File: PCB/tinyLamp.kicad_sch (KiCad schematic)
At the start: 54 parts, among them J1 USB_B_Mini, J2 Conn_02x03_Odd_Even, Q1 Q_NPN_BCE, Q2 Q_NPN_BCE, Q3 Q_NPN_BCE, Q4 Q_NPN_BCE, SW1 SW_Push, SW2 SW_Push, SW3 SW_Push, U1 TP4056, U2 ATtiny13A-SS, X1 BATT+, X2 BATT-

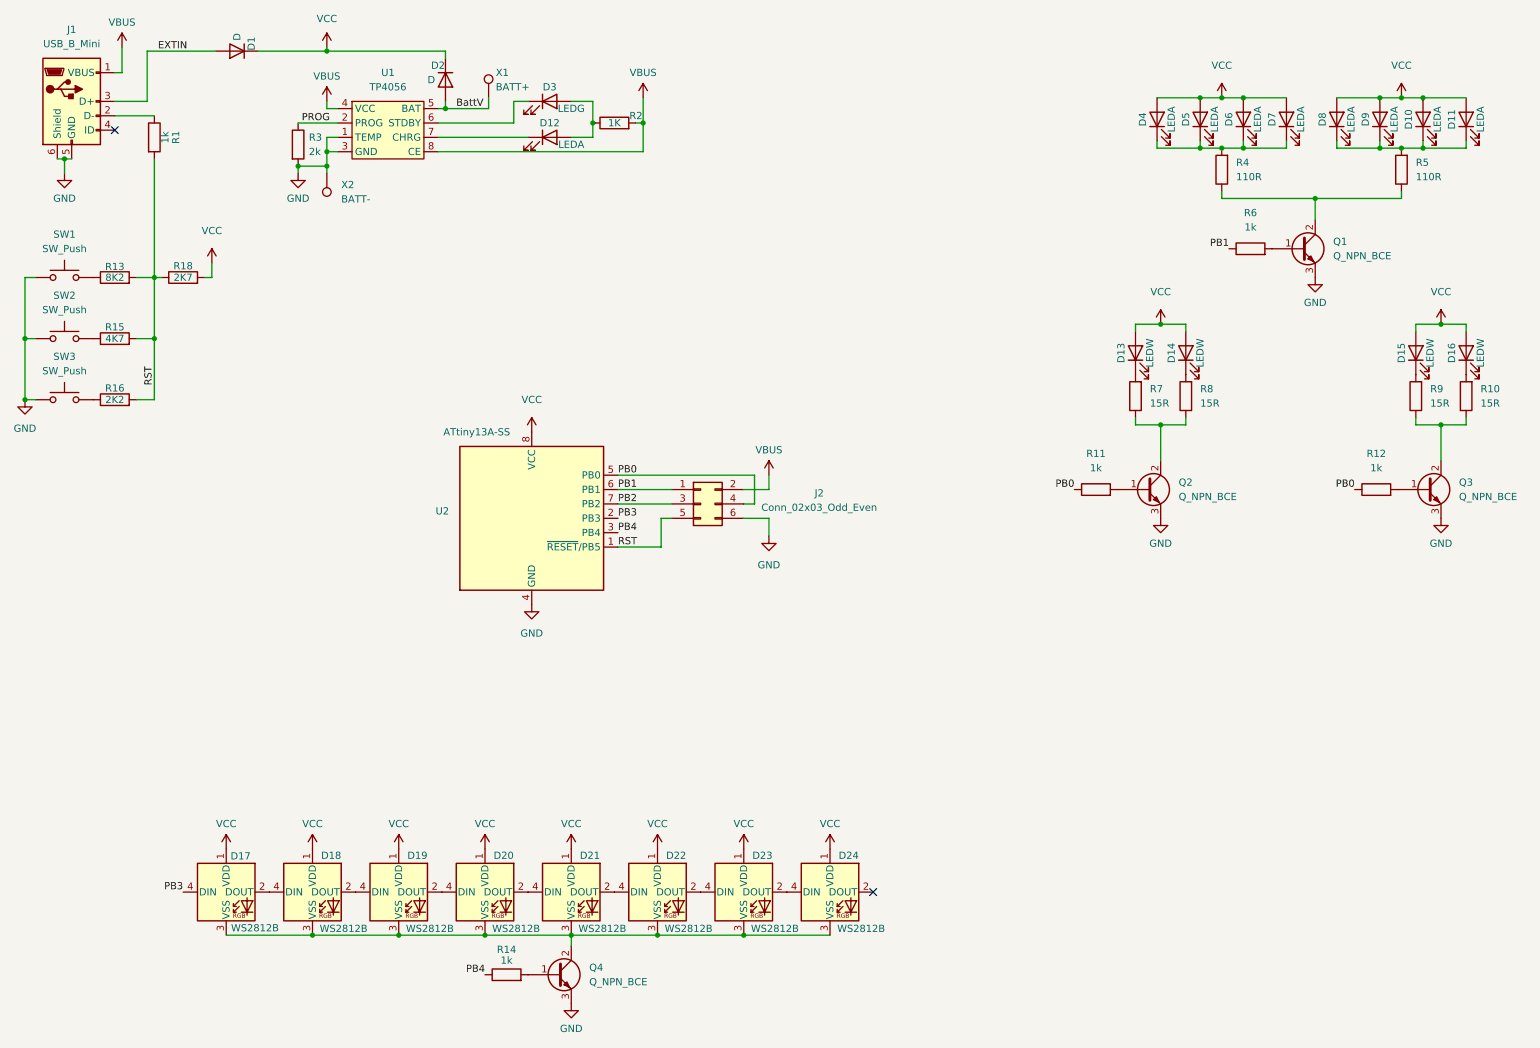
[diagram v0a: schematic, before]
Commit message: made Sub schematics
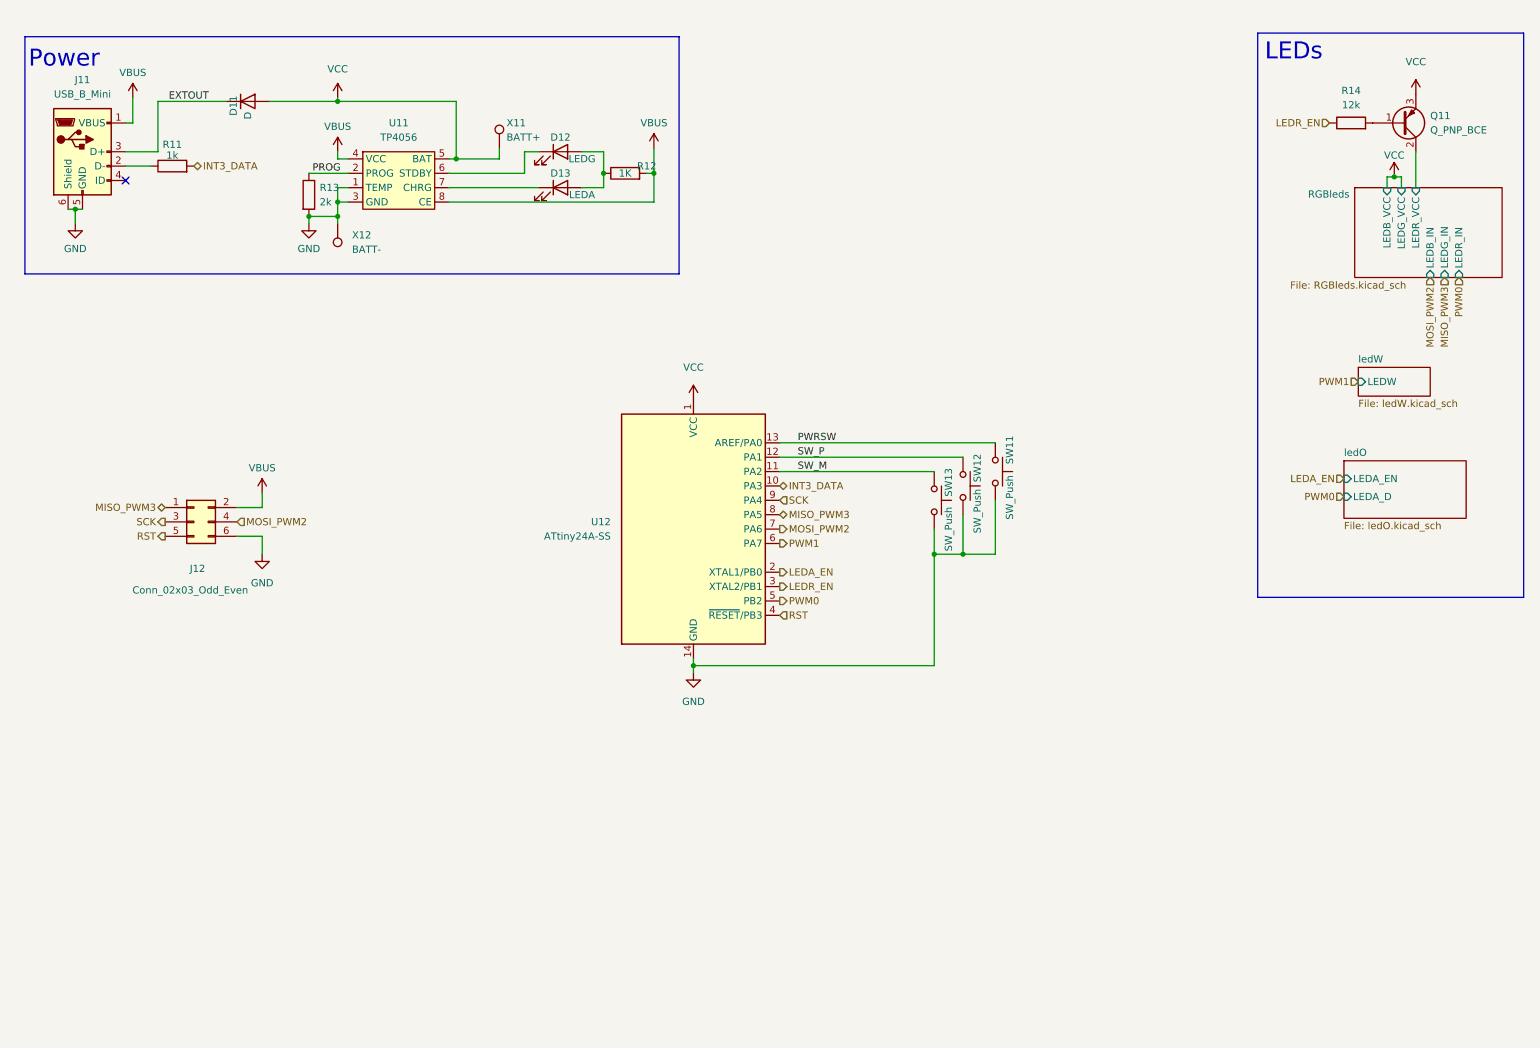
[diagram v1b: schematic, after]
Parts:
- removed D10, D11, D4, D5, D6, D7, D8, D9: LEDA, LED_SMD:LED_0805_2012Metric_Pad1.15x1.40mm_HandSolder, symbol Device:LED
- removed D13, D14, D15, D16: LEDW, LED_SMD:LED_PLCC-2, symbol Device:LED
- removed D17, D18, D19, D20, D21, D22, D23, D24: WS2812B, LED_SMD:LED_WS2812B_PLCC4_5.0x5.0mm_P3.2mm, symbol LED:WS2812B
- removed D2: D, Diode_SMD:D_SOD-123, symbol Device:D
- removed Q1, Q2, Q3, Q4: Q_NPN_BCE, Package_TO_SOT_SMD:SOT-23, symbol Device:Q_NPN_BCE
- removed R10, R7, R8, R9: 15R, Resistor_SMD:R_1206_3216Metric_Pad1.30x1.75mm_HandSolder, symbol Device:R
- removed R11, R12, R6: 1k, Resistor_SMD:R_1206_3216Metric_Pad1.30x1.75mm_HandSolder, symbol Device:R
- removed R13: 8K2, Resistor_SMD:R_1206_3216Metric_Pad1.30x1.75mm_HandSolder, symbol Device:R
- removed R15: 4K7, Resistor_SMD:R_1206_3216Metric_Pad1.30x1.75mm_HandSolder, symbol Device:R
- removed R16: 2K2, Resistor_SMD:R_1206_3216Metric_Pad1.30x1.75mm_HandSolder, symbol Device:R
- removed R18: 2K7, Resistor_SMD:R_1206_3216Metric_Pad1.30x1.75mm_HandSolder, symbol Device:R
- removed R4, R5: 110R, Resistor_SMD:R_1206_3216Metric_Pad1.30x1.75mm_HandSolder, symbol Device:R
- removed U2: ATtiny13A-SS, Package_SO:SOIC-8_3.9x4.9mm_P1.27mm, symbol MCU_Microchip_ATtiny:ATtiny13A-SS
- added Q11: Q_PNP_BCE, Package_TO_SOT_SMD:SOT-23, symbol Device:Q_PNP_BCE
- added U12: ATtiny24A-SS, Package_SO:SOIC-14_3.9x8.7mm_P1.27mm, symbol MCU_Microchip_ATtiny:ATtiny24A-SS
- D11: renamed from D1; footprint Diode_SMD:D_1206_3216Metric_Pad1.42x1.75mm_HandSolder -> Diode_SMD:D_SOD-123
- R14: value 1k -> 12k; Price 0.0021 -> (none)
- renumbered D3 to D12, D12 to D13, J1 to J11, J2 to J12, R1 to R11, R2 to R12, R3 to R13, SW1 to SW11, SW2 to SW12, SW3 to SW13, U1 to U11, X1 to X11, X2 to X12
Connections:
- net BattV is gone; now on net VCC: U11.5 (BAT), X11.1
- net GND: now also SW11.2, SW12.2, SW13.2, U12.14 (GND); no longer SW11.1, SW12.1, SW13.1
- net RST: now also U12.4 (~{RESET}/PB3); no longer R11.2
- net VCC: now also D11.2 (A), Q11.3 (E), U12.1 (VCC); no longer D11.1 (K)
- net at R14.2: now also Q11.1 (B)
- net EXTIN renamed EXTOUT
- net EXTOUT: now also D11.1 (K); no longer D11.2 (A)
- net PB0 renamed MOSI_PWM2
- net MOSI_PWM2: now also U12.7 (PA6)
- net PB1 renamed MISO_PWM3
- net MISO_PWM3: now also U12.8 (PA5)
- net PB2 renamed SCK
- net SCK: now also U12.9 (PA4)
- net PB4 renamed LEDR_EN
- net LEDR_EN: now also U12.3 (XTAL2/PB1)
- new net INT3_DATA: R11.2, U12.10 (PA3)
- new net LEDA_EN: U12.2 (XTAL1/PB0)
- new net PWM0: U12.5 (PB2)
- new net PWM1: U12.6 (PA7)
- new net PWRSW: SW11.1, U12.13 (AREF/PA0)
- new net RGBleds/LEDR_VCC: Q11.2 (C)
- new net SW_M: SW13.1, U12.11 (PA2)
- new net SW_P: SW12.1, U12.12 (PA1)
- no-connect marks 2 -> 1
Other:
- added sheet RGBleds (RGBleds.kicad_sch)
- added sheet ledO (ledO.kicad_sch)
- added sheet ledW (ledW.kicad_sch)
- note added: "LEDs"
- note added: "Power"
- moved on the sheet: D11, D12, D13, J11, J12, R11, R12, R13, SW11, SW12, SW13, U11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
